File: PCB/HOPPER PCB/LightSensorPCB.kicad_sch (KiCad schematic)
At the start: 18 parts, among them J1 Hopper, U1 LTR-329ALS-01, U2 LSM6DSMTR, U3 VL53L3CXV0DH/1

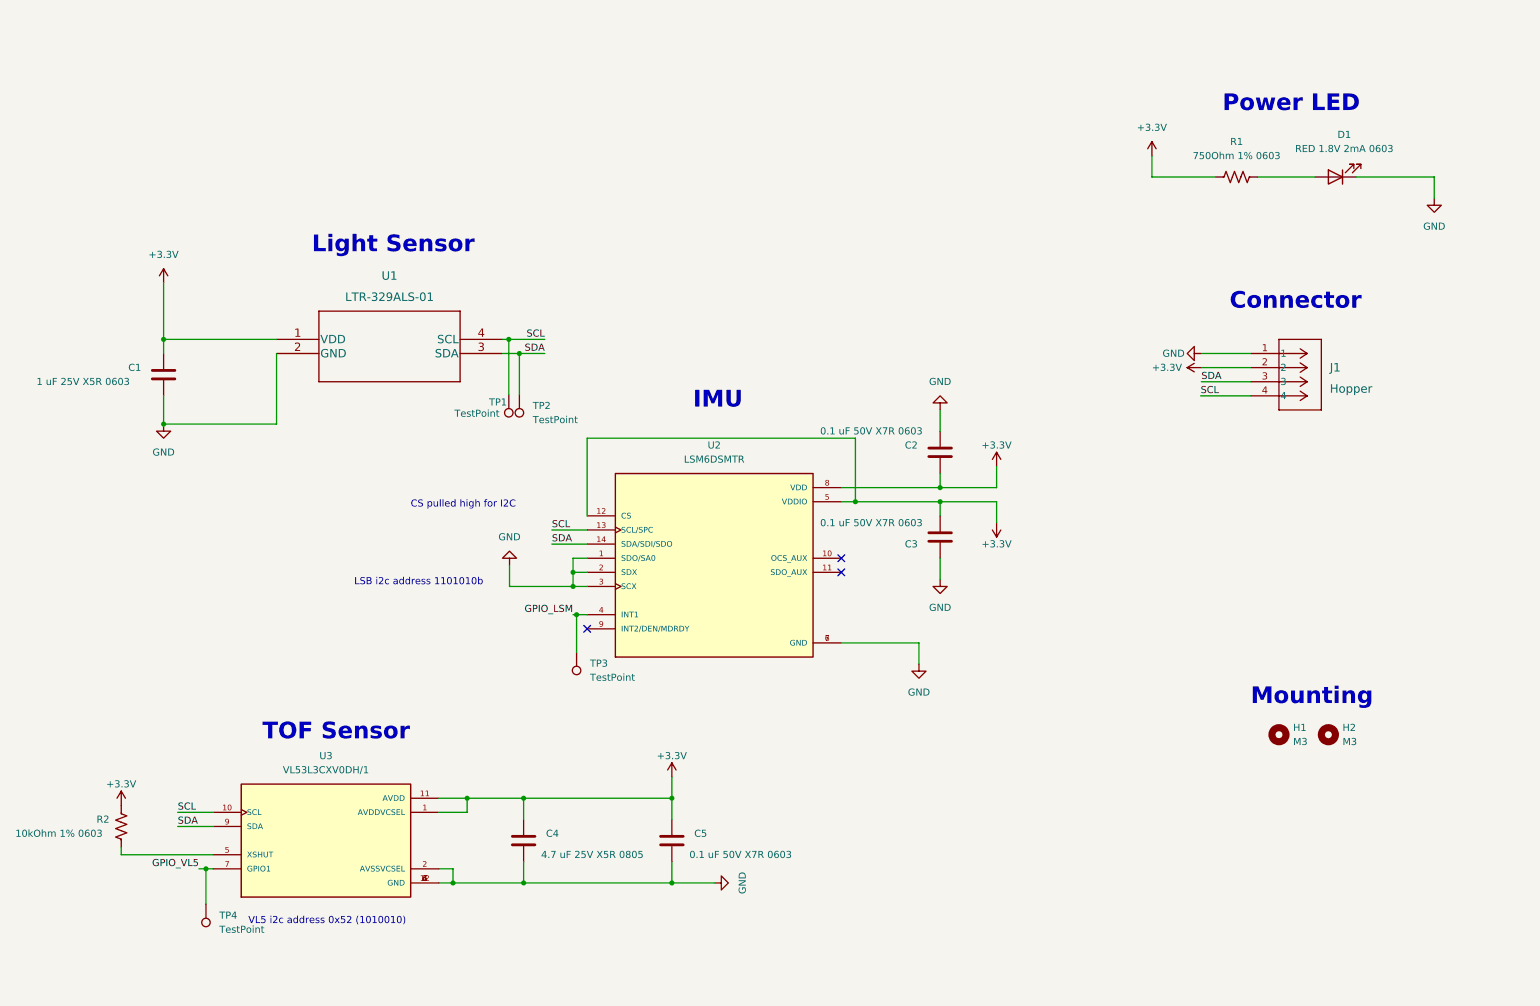
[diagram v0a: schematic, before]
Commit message: PCB - Hopper PCB reviewed and gerbers generated
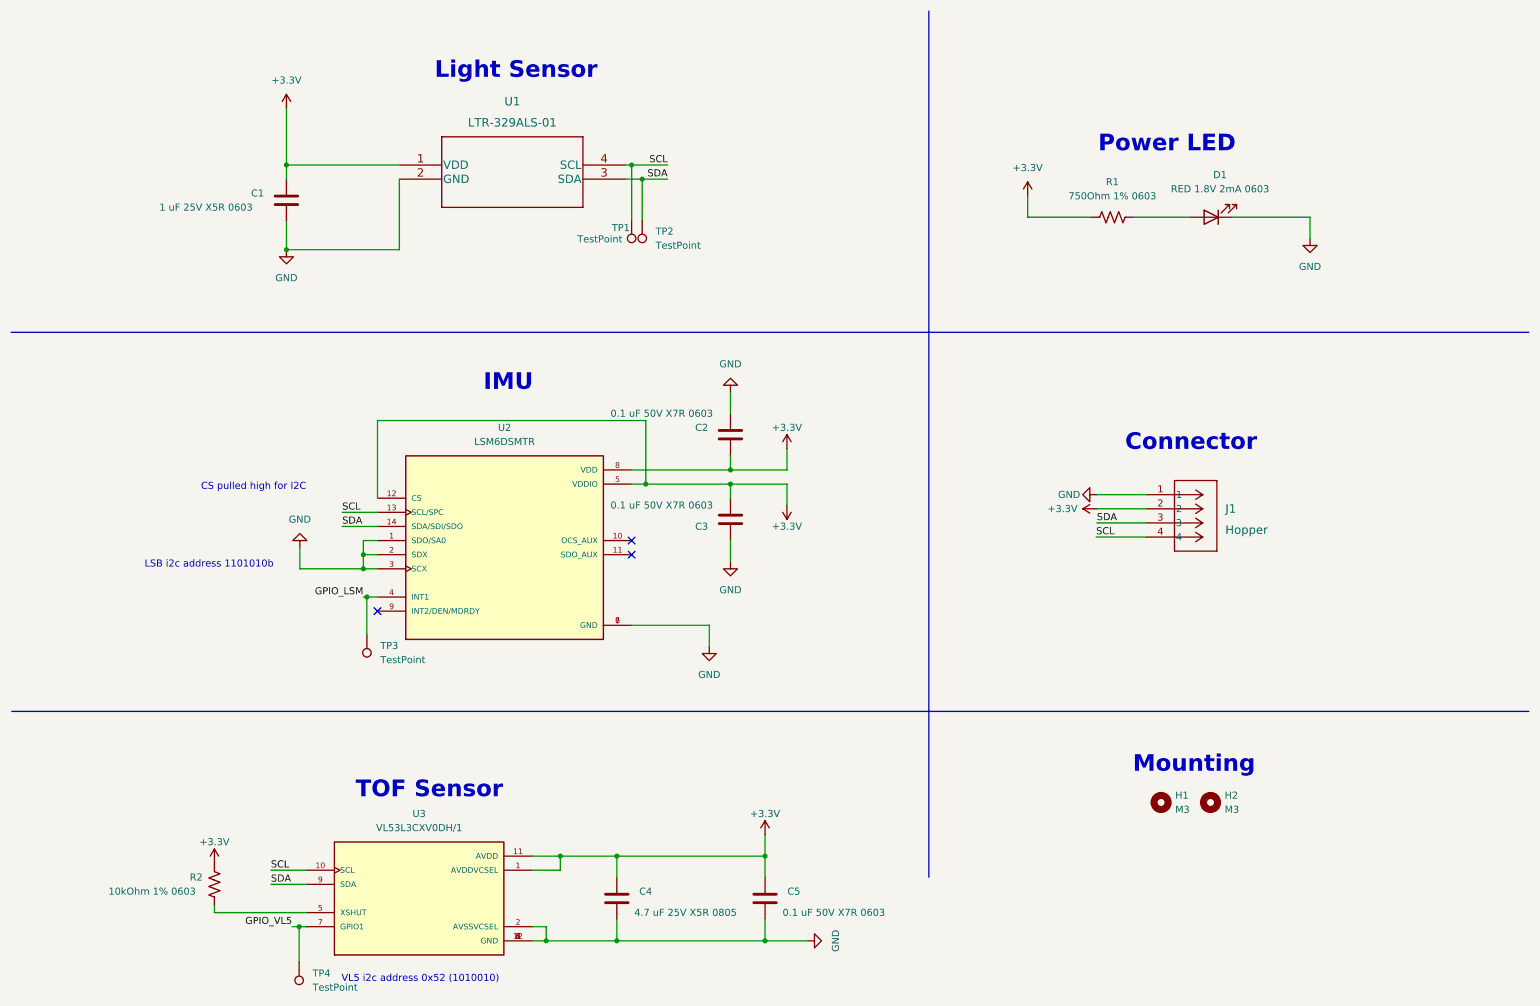
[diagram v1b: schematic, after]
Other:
- moved on the sheet: C1, C2, C3, C4, C5, D1, H1, H2, J1, R1, R2, TP1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
